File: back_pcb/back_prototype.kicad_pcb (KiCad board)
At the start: 2 copper layers, 40 x 100 mm, 84 parts, among them P1 EXPANSION_LEFT, P2 EXPANSION_BOTTOM, P3 EXPANSION_TOP, P4 USB_A, P5 CONN_01X04, P6 ATMEGA_HEADER, P7 EXPANSION_BOTTOM2, P8 CONN_01X02, Q1 Q_PMOS_GSD, Q2 Q_NMOS_GSD, Q3 Q_NMOS_GSD, Q4 Q_PMOS_GSD, U1 PI ZERO, U2 SIM800_BREAKOUT, U3 MCP23017, U4 TP4056_BREAKOUT, U5 RTC, U6 DC_DC_BREAKOUT, Y1 Crystal_Small

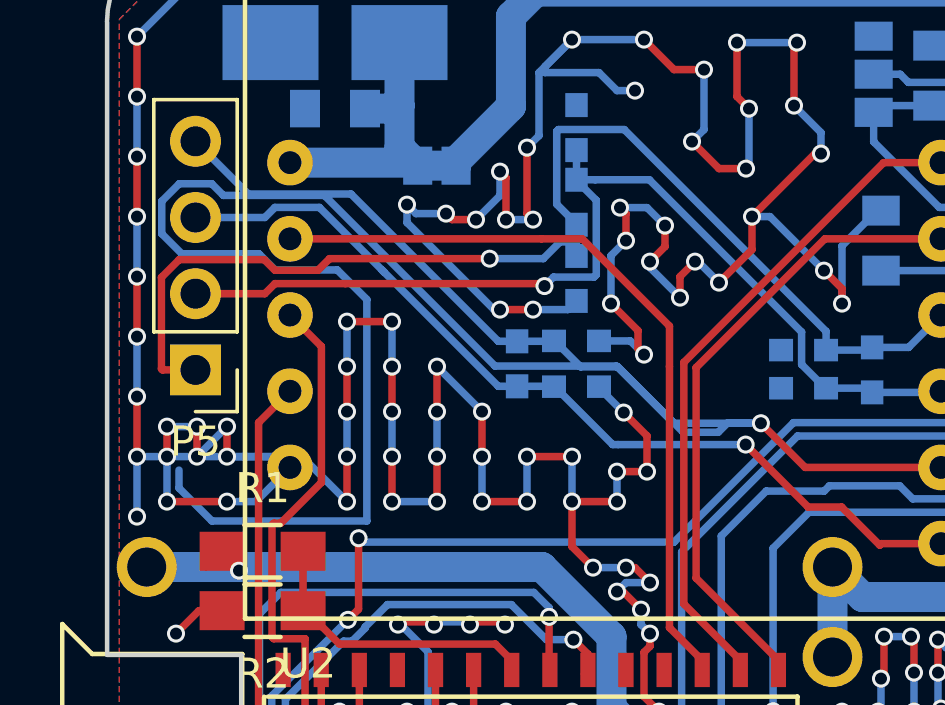
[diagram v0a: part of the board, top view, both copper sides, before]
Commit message: OpenGL router fuckup
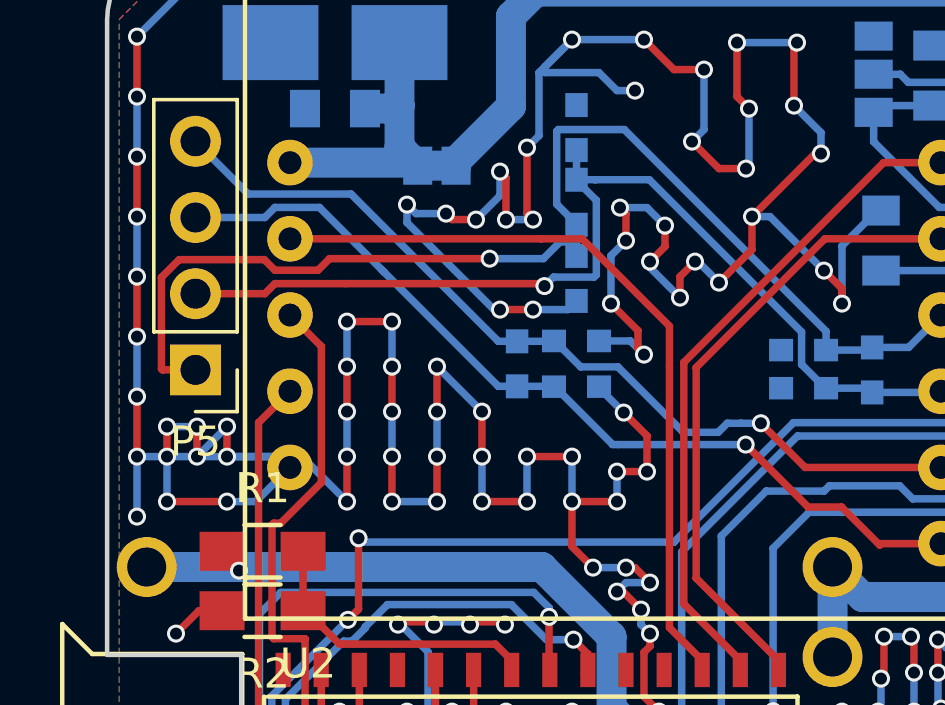
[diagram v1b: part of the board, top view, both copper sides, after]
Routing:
- net SPK+: track 76.9 -> 29.9 mm
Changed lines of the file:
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@@
     (thickness 1.6)
     (drawings 22)
-    (tracks 1845)
+    (tracks 1827)
     (zones 0)
     (modules 84)
@@
   )
   (setup
-    (last_trace_width 0.25)
+    (last_trace_width 0.1)
     (user_trace_width 0.2)
     (user_trace_width 0.25)
@@
     (fp_line (start 1 -1) (end -1 -1) (layer B.CrtYd) (width 0.05))
     (fp_line (start -1 -1) (end -1 1) (layer B.CrtYd) (width 0.05))
-    (pad 1 smd rect (at 0 1.5 360) (size 1 1.5) (layers B.Cu B.Mask)
+    (pad 1 smd rect (at 0 1.5) (size 1 1.5) (layers B.Cu B.Mask)
       (net 52 "Net-(U3-Pad23)"))
   )
@@
   (segment (start 66.8648 55.2196) (end 67.0052 55.36) (width 0.25) (layer B.Cu) (net 15))
   (segment (start 57.15 48.247) (end 57.15 48.272) (width 0.25) (layer B.Cu) (net 15))
-  (segment (start 60.389202 56.388) (end 58.483001 54.481799) (width 0.25) (layer B.Cu) (net 16))
-  (segment (start 44.996801 59.645799) (end 43.90001 58.549008) (width 0.25) (layer B.Cu) (net 16))
-  (segment (start 43.909999 48.404999) (end 43.324999 48.989999) (width 0.25) (layer B.Cu) (net 16))
-  (segment (start 63.2968 56.388) (end 60.389202 56.388) (width 0.25) (layer B.Cu) (net 16))
-  (segment (start 58.483001 54.481799) (end 54.434498 54.481799) (width 0.25) (layer B.Cu) (net 16))
-  (segment (start 54.434498 54.481799) (end 48.746888 48.794189) (width 0.25) (layer B.Cu) (net 16))
-  (segment (start 47.101839 51.278201) (end 49.175841 51.278201) (width 0.25) (layer B.Cu) (net 16))
-  (segment (start 48.746888 48.794189) (end 45.379191 48.794189) (width 0.25) (layer B.Cu) (net 16))
-  (segment (start 49.175841 51.278201) (end 50.161601 52.263961) (width 0.25) (layer B.Cu) (net 16))
-  (segment (start 45.379191 48.794189) (end 44.990001 48.404999) (width 0.25) (layer B.Cu) (net 16))
-  (segment (start 46.562599 50.738961) (end 47.101839 51.278201) (width 0.25) (layer B.Cu) (net 16))
-  (segment (start 44.990001 48.404999) (end 43.909999 48.404999) (width 0.25) (layer B.Cu) (net 16))
-  (segment (start 50.161601 52.263961) (end 50.161601 59.645799) (width 0.25) (layer B.Cu) (net 16))
-  (segment (start 43.324999 48.989999) (end 43.324999 50.070001) (width 0.25) (layer B.Cu) (net 16))
-  (segment (start 43.324999 50.070001) (end 43.993959 50.738961) (width 0.25) (layer B.Cu) (net 16))
-  (segment (start 50.161601 59.645799) (end 44.996801 59.645799) (width 0.25) (layer B.Cu) (net 16))
-  (segment (start 43.993959 50.738961) (end 46.562599 50.738961) (width 0.25) (layer B.Cu) (net 16))
-  (segment (start 43.90001 58.549008) (end 43.90001 57.950992) (width 0.25) (layer B.Cu) (net 16))
   (segment (start 63.2968 56.388) (end 64.77 57.8612) (width 0.25) (layer F.Cu) (net 16))
   (segment (start 64.77 57.8612) (end 69.2996 57.8612) (width 0.25) (layer F.Cu) (net 16))

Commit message: Added component values to the back PCB - for BOM
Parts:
- C13, C14, C15, C25, C5, C6, C7, C8: value C_Small -> 100nF
- C16, C17, C18, C19, C20, C21: value C_Small -> 10pF
- C22, C23, C24: value C_Small -> 33pF
- C4: value C_Small -> 10uF
- D1: value D_Small -> SS14
- D3: value Led_RGB_CA -> Led_RGB_CA_CC
- JP3: value JUMPER3 -> A0
- JP4: value JUMPER3 -> A1
- JP6: value JUMPER3 -> A2
- JP7: value JUMPER3 -> 3V3/5V
- JP8: value JUMPER3 -> CA/CC
- P5: value CONN_01X04 -> AUDIO_CONN
- Q1, Q4: value Q_PMOS_GSD -> IRLML6401
- Q2, Q3: value Q_NMOS_GSD -> BSS138
- R1, R10, R11, R2, R3, R8, R9: value R -> 10K
- R5, R6, R7: value R -> 1K
- Y1: value Crystal_Small -> 32.768Hz
